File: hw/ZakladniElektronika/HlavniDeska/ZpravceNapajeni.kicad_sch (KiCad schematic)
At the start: 12 parts, among them Q10 Q_PMOS_DGS-P, Q13 Q_PMOS_DGS-P

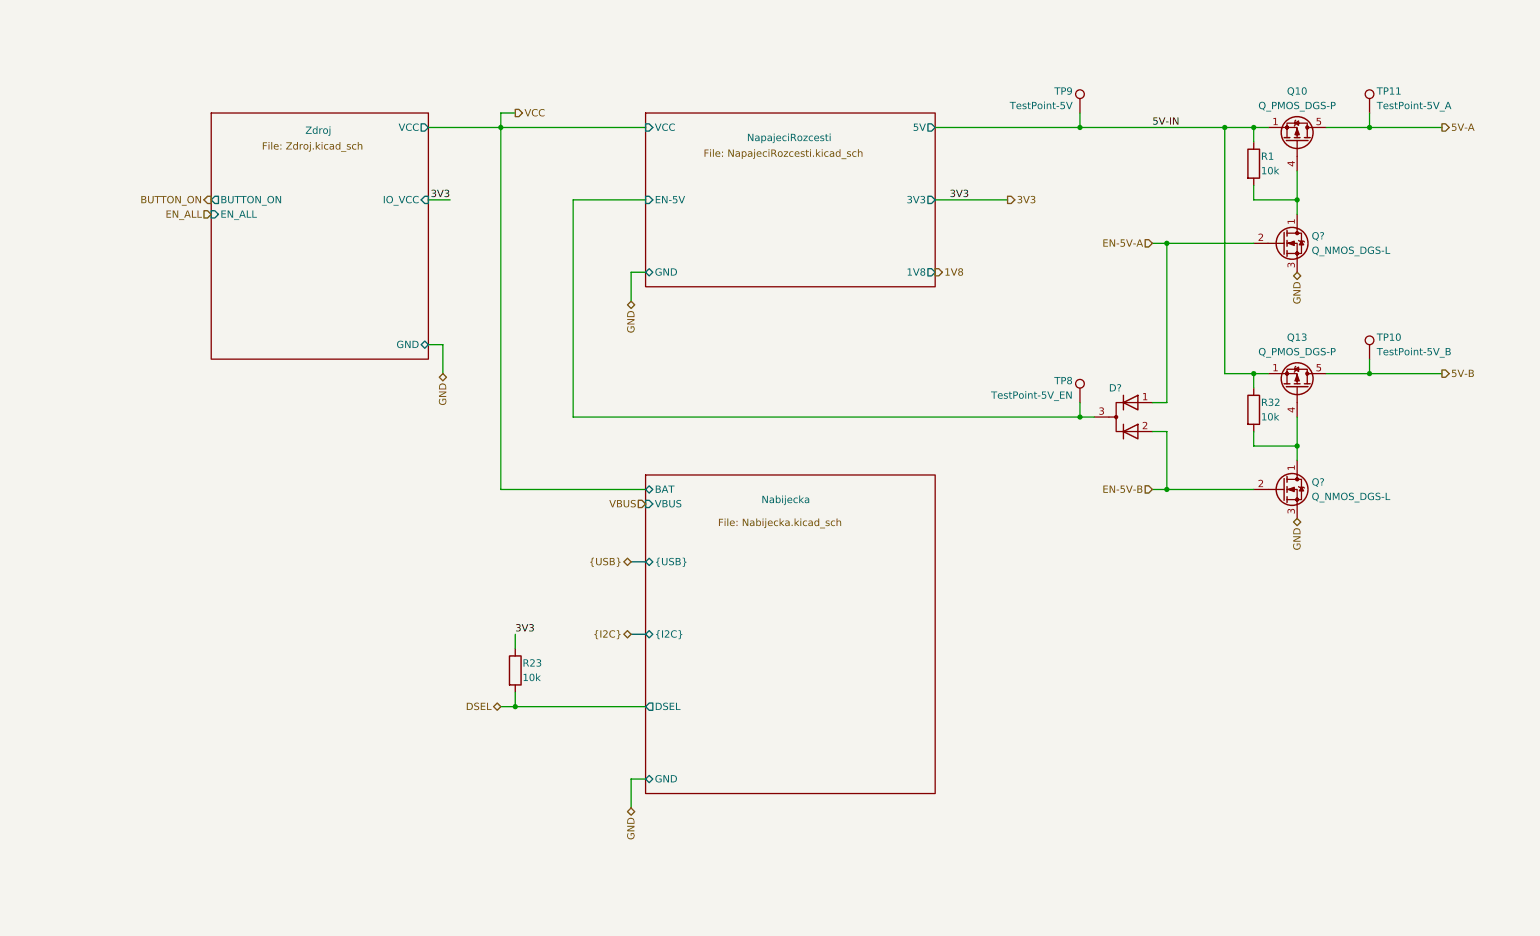
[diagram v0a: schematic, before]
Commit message: Hw wip
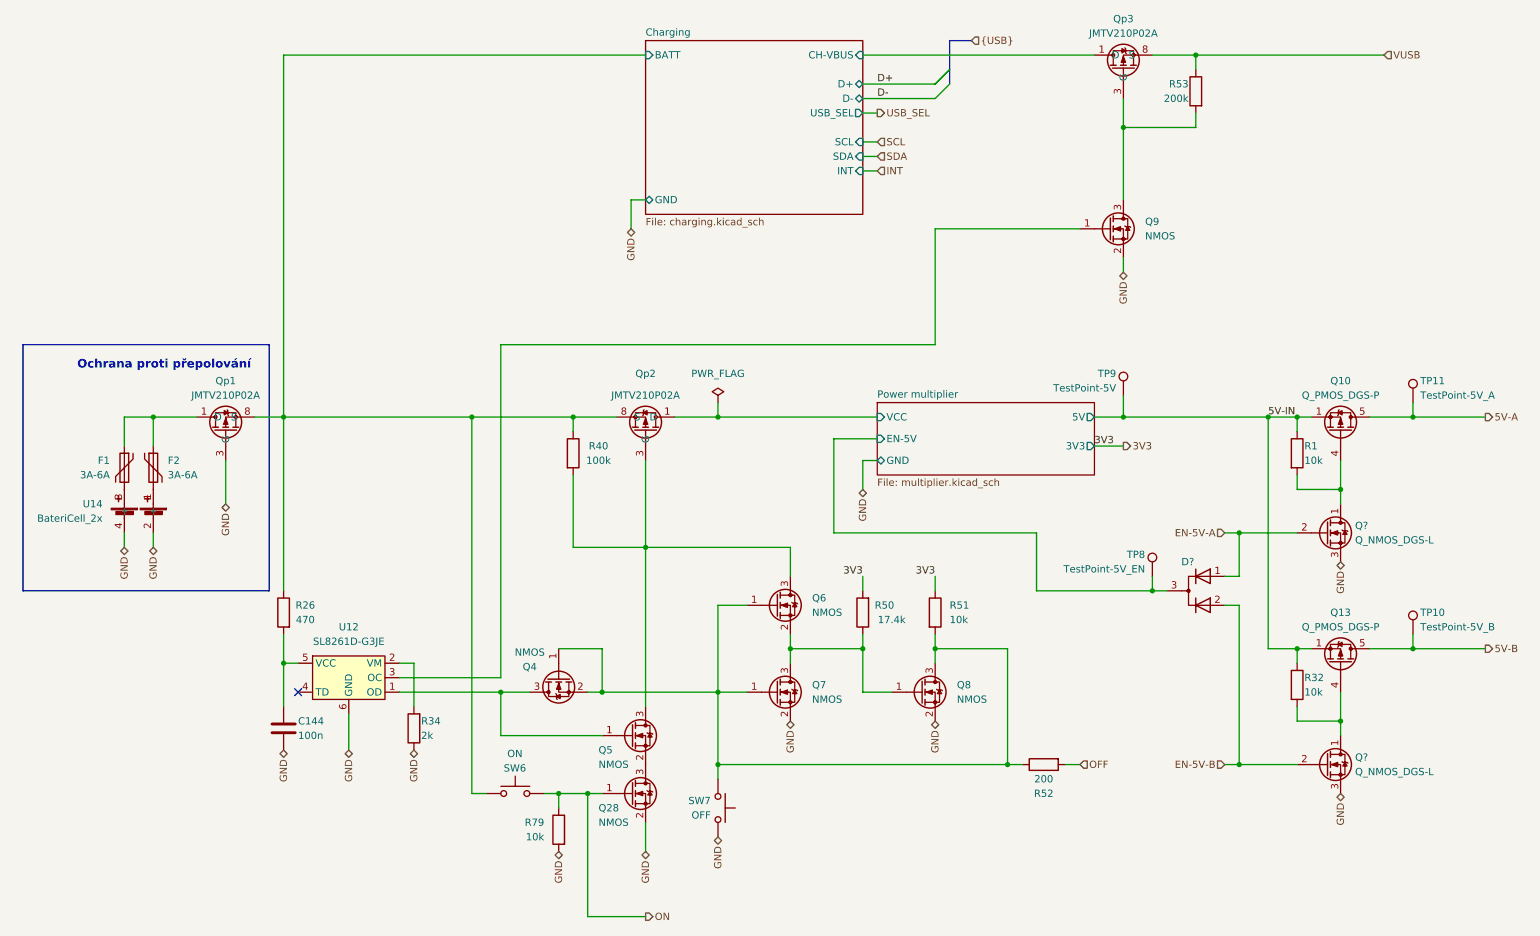
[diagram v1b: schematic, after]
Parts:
- removed R23: 10k, Resistor_SMD:R_0402_1005Metric, symbol Device:R
- added C144: 100n, Capacitor_SMD:C_0402_1005Metric, symbol Device:C
- added F1, F2: 3A-6A, Inductor_SMD:L_1206_3216Metric, symbol Device:Polyfuse
- added Q28, Q4, Q5, Q6, Q7, Q8, Q9: NMOS, Package_TO_SOT_SMD:SOT-723, symbol Device:Q_NMOS_GSD
- added Qp1, Qp2, Qp3: JMTV210P02A, Package_DFN_QFN:Diodes_UDFN2020-6_Type-F, symbol RKL-MOSFET:JMTV210P02A
- added R26: 470, Resistor_SMD:R_0402_1005Metric, symbol Device:R
- added R34: 2k, Resistor_SMD:R_0402_1005Metric, symbol Device:R
- added R40: 100k, Resistor_SMD:R_0402_1005Metric, symbol Device:R
- added R50: 17.4k, Resistor_SMD:R_0402_1005Metric, symbol Device:R
- added R51, R79: 10k, Resistor_SMD:R_0402_1005Metric, symbol Device:R
- added R52: 200, Resistor_SMD:R_0402_1005Metric, symbol Device:R
- added R53: 200k, Resistor_SMD:R_0402_1005Metric, symbol Device:R
- added SW6: ON, Button_Switch_SMD:SW_Push_1P1T_NO_Vertical_Wuerth_434133025816, symbol Switch:SW_Push
- added SW7: OFF, Button_Switch_SMD:SW_Push_1P1T_NO_Vertical_Wuerth_434133025816, symbol Switch:SW_Push
- added U12: SL8261D-G3JE, Package_TO_SOT_SMD:SOT-23-6, symbol RKL-BatteryManager:DW01A
- added U14: BateriCell_2x, RKL-Batteries:2x18650-holder-jlc_SMD-typ, symbol RKL-BatteryManager:BateriCell_2x
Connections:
- net 3V3: now also R50.2, R51.1
- net GND: now also C144.2, Q28.2 (S), Q7.2 (S), Q8.2 (S), Q9.2 (S), Qp1.3 (G), R34.1, R79.2, SW7.1, U12.6 (GND), U14.2 (-), U14.4 (-)
- net NapajeciRozcesti/EN-5V renamed Power multiplier/EN-5V
- new net: Q4.3 (D), Q5.1 (G), U12.1 (OD)
- new net: R34.2, U12.2 (VM)
- new net: Q9.1 (G), U12.3 (OC)
- new net: C144.1, R26.2, U12.5 (VCC)
- new net: Q4.1 (G), Q4.2 (S), Q6.1 (G), Q7.1 (G), Q8.3 (D), R51.2, R52.1, SW7.2
- new net: Q6.2 (S), Q7.3 (D), Q8.1 (G), R50.1
- new net: Q5.3 (D), Q6.3 (D), Qp2.3 (G), R40.2
- new net: Q28.3 (D), Q5.2 (S)
- new net: F1.1, F2.1, Qp1.1 (D), Qp1.2 (D), Qp1.5 (D), Qp1.6 (D), Qp1.7 (D)
- new net: F1.2, U14.3 (+)
- new net: Q9.3 (D), Qp3.3 (G), R53.2
- new net: F2.2, U14.1 (+)
- new net Charging/BATT: Qp1.4 (S), Qp1.8 (S), Qp2.4 (S), Qp2.8 (S), R26.1, R40.1, SW6.1
- new net Charging/CH-VBUS: Qp3.1 (D), Qp3.2 (D), Qp3.5 (D), Qp3.6 (D), Qp3.7 (D)
- new net OFF: R52.2
- new net ON: Q28.1 (G), R79.1, SW6.2
- new net Power multiplier/VCC: Qp2.1 (D), Qp2.2 (D), Qp2.5 (D), Qp2.6 (D), Qp2.7 (D)
- new net VUSB: Qp3.4 (S), Qp3.8 (S), R53.1
- no-connect marks 0 -> 1
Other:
- removed sheet Nabijecka
- removed sheet NapajeciRozcesti
- removed sheet Zdroj
- added sheet Charging (charging.kicad_sch)
- added sheet Power multiplier (multiplier.kicad_sch)
- note added: "Ochrana proti přepolování"
- moved on the sheet: D?, Q10, Q13, Q?, R1, R32, TP10, TP11, TP8, TP9
